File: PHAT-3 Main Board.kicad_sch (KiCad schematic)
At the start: 17 parts, among them K1 G5LE-1, P1 Power Terminal Block, P2 Power Terminal Block, P3 Power Terminal Block, P4 Power Terminal Block, U1 AHT21, U10 Logic Level Converter, U2 ESP32-S3 Dual-core SX1262, U3 BME280, U4 GY-521 MPU-6050, U5 LM2596, U6 GT-7U, U7 SCD41, U8 uCAM-III, U9 SD Card Reader

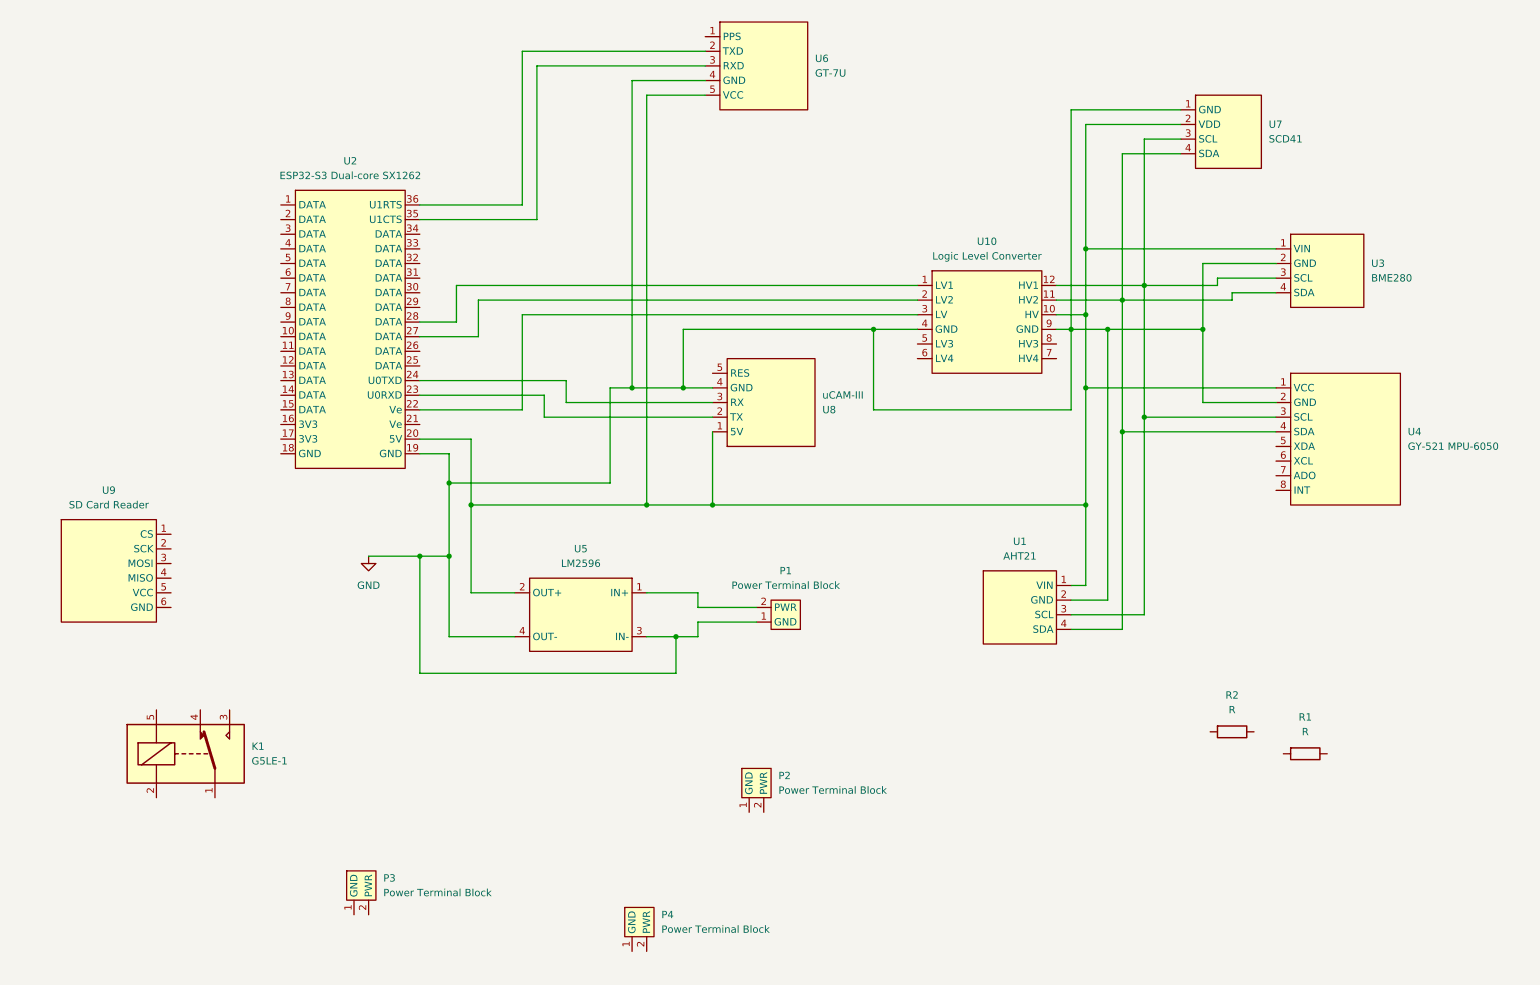
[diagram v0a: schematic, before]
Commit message: First Wiring Draft
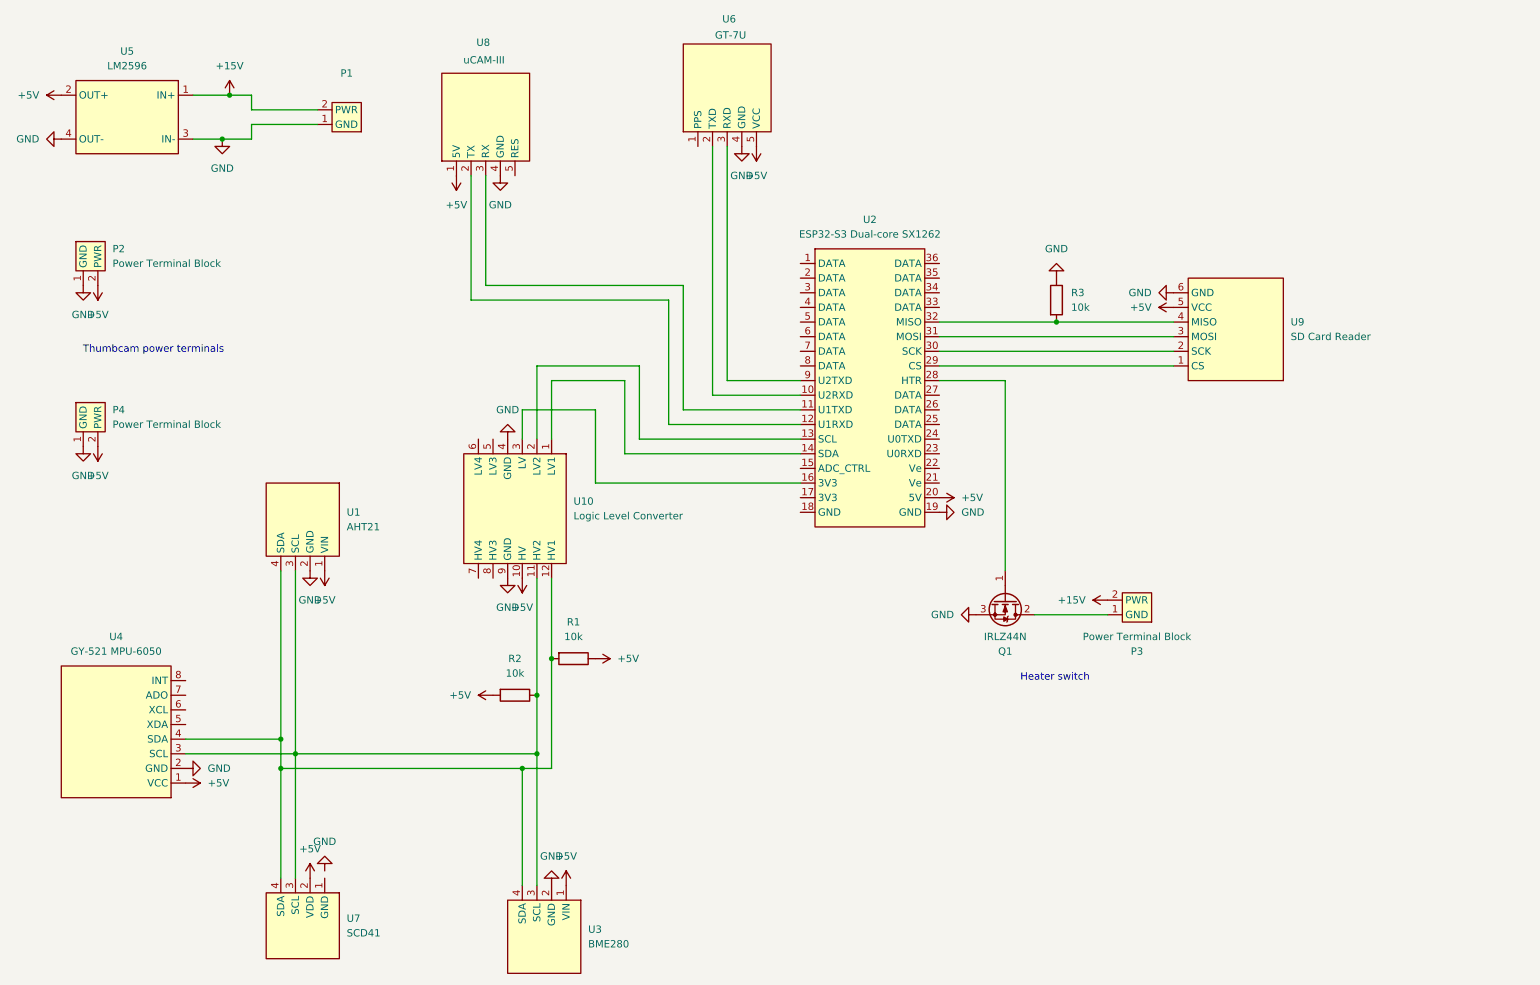
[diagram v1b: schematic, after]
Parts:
- removed K1: G5LE-1, Relay_THT:Relay_SPDT_Omron-G5LE-1, symbol Relay:G5LE-1
- added Q1: IRLZ44N, Package_TO_SOT_THT:TO-220-3_Vertical, symbol Transistor_FET:IRLZ44N
- added R3: 10k, Resistor_THT:R_Axial_DIN0207_L6.3mm_D2.5mm_P10.16mm_Horizontal, symbol Device:R
- R1, R2: value R -> 10k
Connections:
- net GND: now also P2.1 (GND), P4.1 (GND), U9.6 (GND), Q1.3 (S), R3.1; no longer U7.1 (GND)
- net at U6.2 (TXD): now also U2.10 (U2RXD); no longer U2.36 (U1RTS)
- net at U6.3 (RXD): now also U2.9 (U2TXD); no longer U2.35 (U1CTS)
- net +5V: now reaches U1.1 (VIN), U10.10 (HV), U2.20 (5V), U3.1 (VIN), U4.1 (VCC), U5.2 (OUT+), U6.5 (VCC), U7.2 (VDD), U8.1 (5V)
- net +5V: now also P2.2 (PWR), P4.2 (PWR), R1.1, R2.2, U9.5 (VCC)
- net at R2.1: now also U1.3 (SCL), U10.11 (HV2), U3.3 (SCL), U4.3 (SCL), U7.3 (SCL)
- net at U1.4 (SDA), U3.4 (SDA), U4.4 (SDA)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: now also R1.2, U10.12 (HV1); no longer U10.11 (HV2)
- net at U9.1 (CS): now also U2.29 (CS)
- net at U9.2 (SCK): now also U2.30 (SCK)
- net at U9.3 (MOSI): now also U2.31 (MOSI)
- net at U9.4 (MISO): now also U2.32 (MISO), R3.2
- net +15V: now reaches P1.2 (PWR), U5.1 (IN+)
- net +15V: now also P3.2 (PWR)
- net at U2.11 (U1TXD): now also U8.3 (RX)
- net at U2.12 (U1RXD): now also U8.2 (TX)
- net at U2.13 (SCL): now also U10.2 (LV2)
- net at U2.14 (SDA): now also U10.1 (LV1)
- net at U2.16 (3V3): now also U10.3 (LV)
- net at U2.22 (Ve): no longer U10.3 (LV)
- net at U2.23 (U0RXD): no longer U8.2 (TX)
- net at U2.24 (U0TXD): no longer U8.3 (RX)
- net at U2.27 (DATA): no longer U10.2 (LV2)
- net at U2.28 (HTR): now also Q1.1 (G); no longer U10.1 (LV1)
- net at P3.1 (GND): now also Q1.2 (D)
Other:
- note added: "Heater switch"
- note added: "Thumbcam power terminals"
- moved on the sheet: P1, P2, P3, P4, R1, R2, U1, U10, U2, U3, U4, U5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
